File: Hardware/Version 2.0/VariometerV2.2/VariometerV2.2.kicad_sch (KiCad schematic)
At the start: 129 parts, among them IC1 TP4056, IC2 MAX809STRG, IC3 TPS73701DCQR, IC4 TPS22916CNYFPR, IC5 ESP32-S3-WROOM, J1 LED_CHRG, J10 Conn_01x02, J11 Conn_01x02, J12 TFP09-2-12B, J13 5-1814832-2, J2 LED_STBY, J3 USB_B_Micro, J4 Conn_01x08, J5 Conn_01x02_Male, J6 Conn_01x02, J7 Conn_01x05, J8 Conn_01x02, J9 Conn_01x02, Q1 AO3401A, Q2 AO3401A, Q3 AO3400A, SW1 Switch_SW_Push, SW2 Switch_SW_Push, U1 SRV05-4, U2 SRV05-4, U3 SRV05-4, U4 MAX98357A, U5 QMC5883L, U6 BMI088, U7 ATGM336H-5N31, U8 DPS310

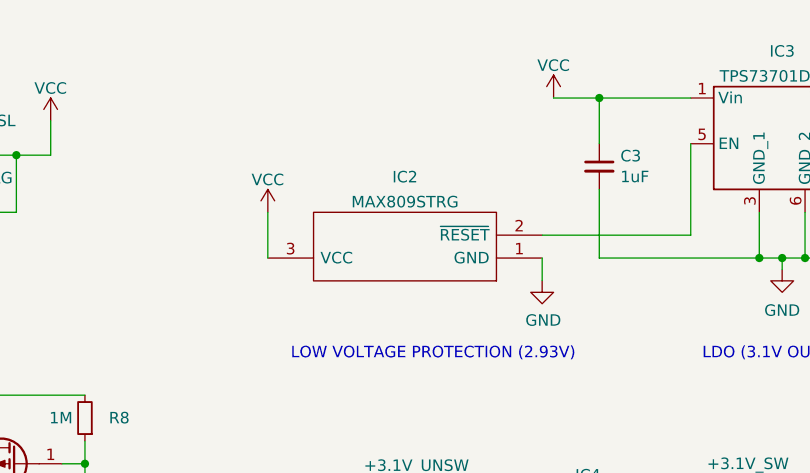
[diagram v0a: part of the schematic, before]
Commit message: Start Board Devlopment
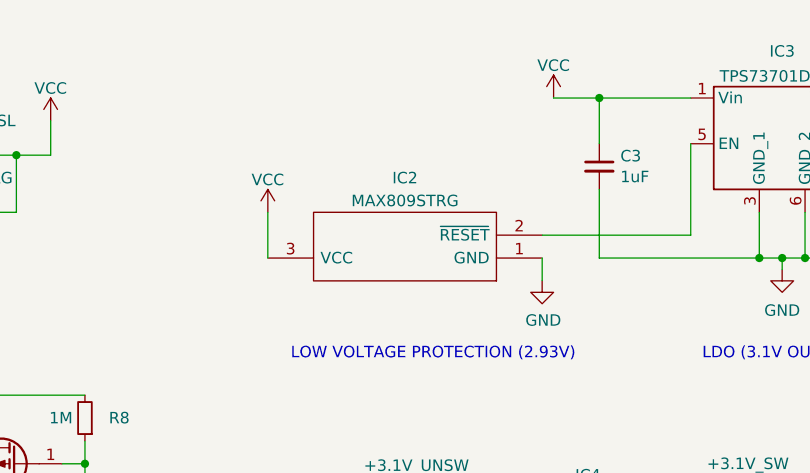
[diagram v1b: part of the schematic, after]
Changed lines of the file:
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@@
   (symbol (lib_id "SamacSys_Parts:MAX809STRG") (at 201.93 39.37 180) (unit 1)
     (in_bom yes) (on_board yes) (dnp no) (fields_autoplaced)
-    (property "Reference" "IC2" (at 186.69 30.3743 0)
+    (property "Reference" "IC2" (at 186.69 30.48 0)
       (effects (font (size 1.27 1.27)))
     )
-    (property "Value" "MAX809STRG" (at 186.69 33.1494 0)
+    (property "Value" "MAX809STRG" (at 186.69 33.02 0)
       (effects (font (size 1.27 1.27)))
     )

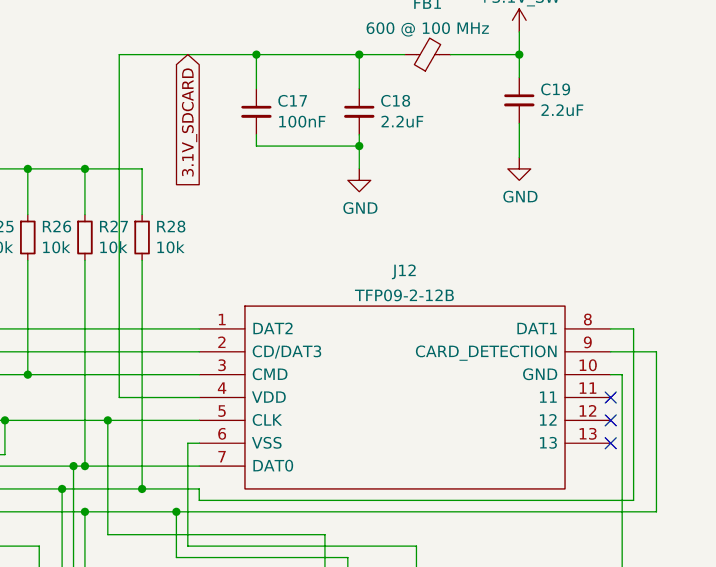
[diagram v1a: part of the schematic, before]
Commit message: Working on PCB
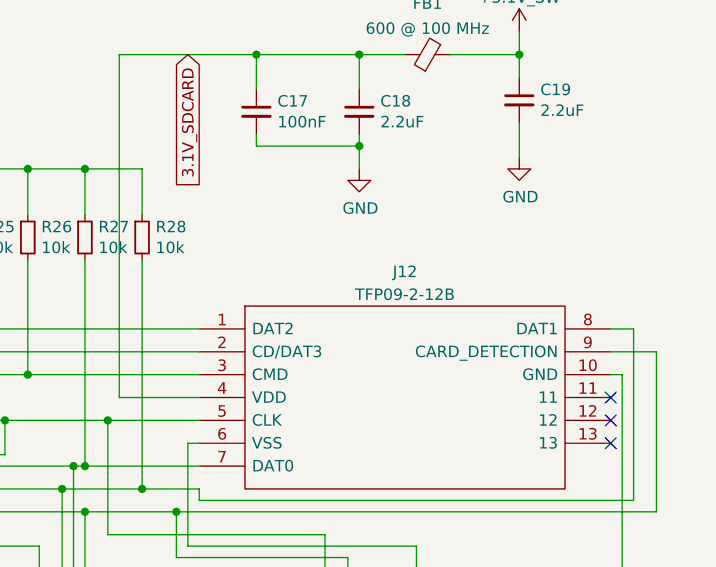
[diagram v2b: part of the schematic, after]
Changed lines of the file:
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@@
   (symbol (lib_name "TFP09-2-12B_1") (lib_id "SamacSys_Parts:TFP09-2-12B") (at 347.98 55.88 0) (unit 1)
     (in_bom yes) (on_board yes) (dnp no) (fields_autoplaced)
-    (property "Reference" "J12" (at 370.84 49.4243 0)
+    (property "Reference" "J12" (at 370.84 49.53 0)
       (effects (font (size 1.27 1.27)))
     )
-    (property "Value" "TFP09-2-12B" (at 370.84 52.1994 0)
+    (property "Value" "TFP09-2-12B" (at 370.84 52.07 0)
       (effects (font (size 1.27 1.27)))
     )
